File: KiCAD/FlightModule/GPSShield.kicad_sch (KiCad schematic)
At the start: 6 parts

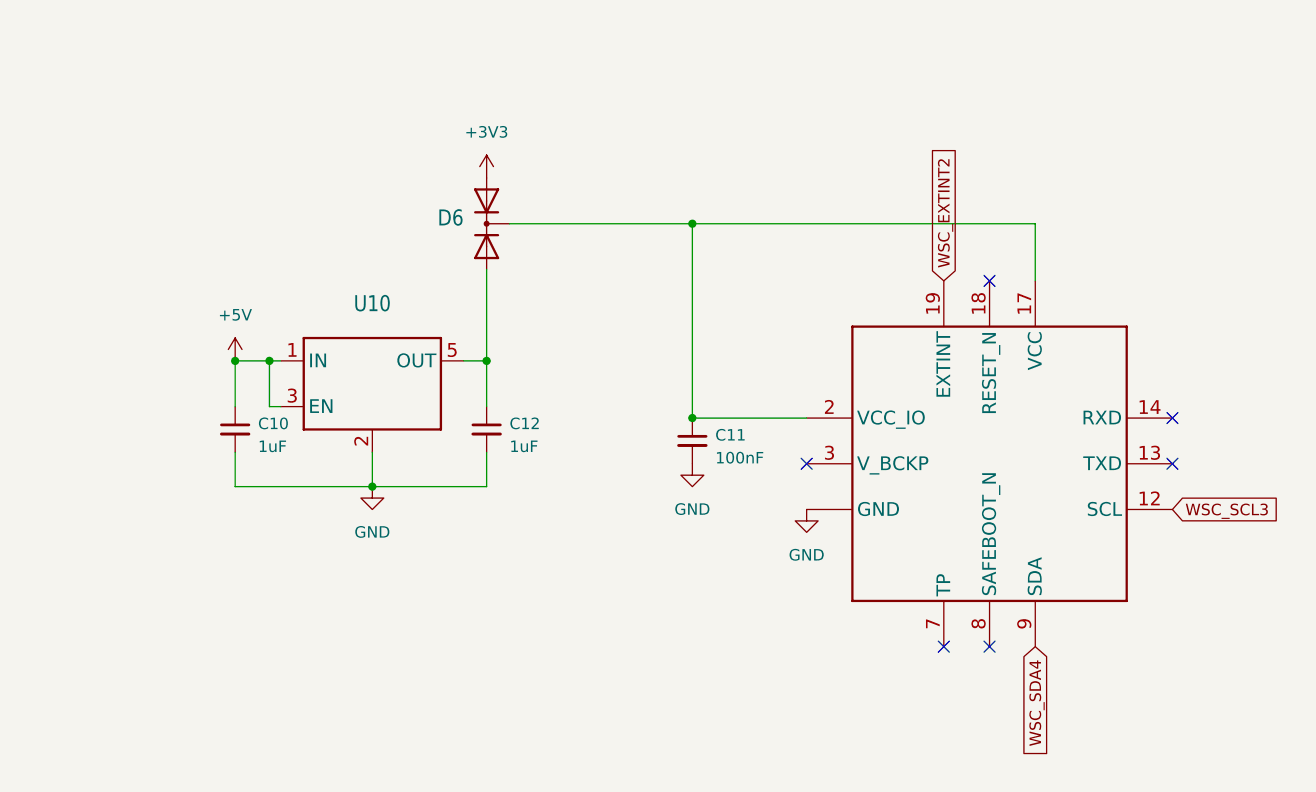
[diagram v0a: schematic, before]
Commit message: GNSSモジュール，SAM-M8Qの回路図完成
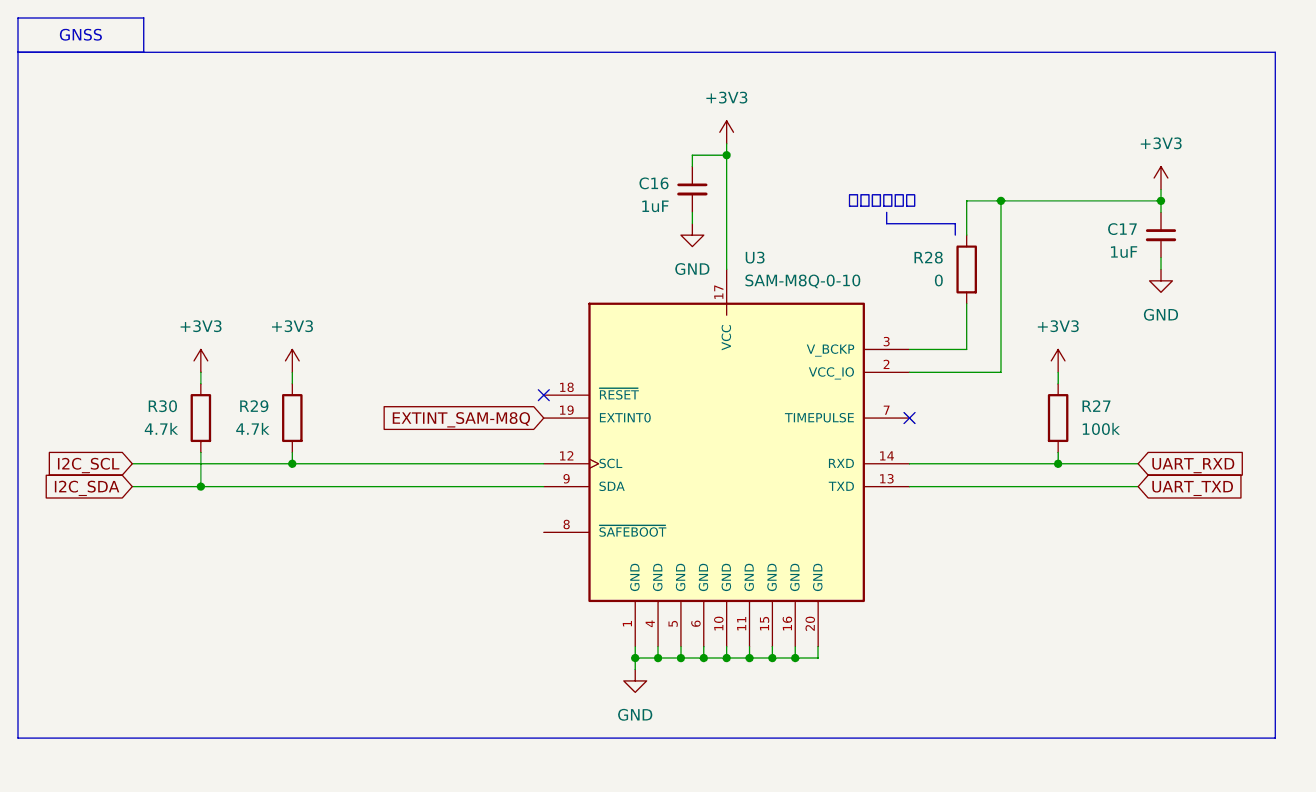
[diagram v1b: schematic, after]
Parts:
- removed C10, C12: 1uF, Capacitor_SMD:C_1206_3216Metric_Pad1.33x1.80mm_HandSolder, symbol Device:C_Small
- removed C11: 100nF, Capacitor_SMD:C_1206_3216Metric_Pad1.33x1.80mm_HandSolder, symbol Device:C_Small
- removed D6: ~, MKRGPSShield_V4.0:SOT65P210X110-3N, symbol MKRGPSShield_V4.0-eagle-import:Arduino-diodes_A2K_SOT-323
- removed IC2: ~, GPSShield:UBLOXLIB_SAM-M8Q, symbol MKRGPSShield_V4.0-eagle-import:SAM-M8Q
- removed U10: ~, MKRGPSShield_V4.0:SOT25, symbol MKRGPSShield_V4.0-eagle-import:AP2112K-3.3
- added C16, C17: 1uF, Capacitor_SMD:C_1206_3216Metric_Pad1.33x1.80mm_HandSolder, symbol Device:C_Small
- added R27: 100k, Resistor_SMD:R_0603_1608Metric_Pad0.98x0.95mm_HandSolder, symbol Device:R
- added R28: 0, Resistor_SMD:R_0603_1608Metric_Pad0.98x0.95mm_HandSolder, symbol Device:R
- added R29, R30: 4.7k, Resistor_SMD:R_0603_1608Metric_Pad0.98x0.95mm_HandSolder, symbol Device:R
- added U3: SAM-M8Q-0-10, TSRP_IC:MODULE_SAM-M8Q-0-10, symbol TSRP_IC:SAM-M8Q-0-10
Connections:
- net +3V3: now also C16.1, C17.1, R27.1, R28.1, R29.1, R30.1, U3.17 (VCC), U3.2 (VCC_IO)
- net GND: now also C16.2, C17.2, U3.1 (GND), U3.10 (GND), U3.11 (GND), U3.15 (GND), U3.16 (GND), U3.20 (GND), U3.4 (GND), U3.5 (GND), U3.6 (GND)
- new net: R28.2, U3.3 (V_BCKP)
- new net EXTINT_SAM-M8Q: U3.19 (EXTINT0)
- new net I2C_SCL: R29.2, U3.12 (SCL)
- new net I2C_SDA: R30.2, U3.9 (SDA)
- new net UART_RXD: R27.2, U3.14 (RXD)
- new net UART_TXD: U3.13 (TXD)
- no-connect marks 6 -> 2
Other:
- note added: "ジャンパ抵抗"

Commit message: 回路図8割完成
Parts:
- U3: footprint TSRP_IC:MODULE_SAM-M8Q-0-10 -> SAM-M8Q-0-10:MODULE_SAM-M8Q-0-10
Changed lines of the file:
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@@
 			)
 		)
-		(property "Footprint" "TSRP_IC:MODULE_SAM-M8Q-0-10"
+		(property "Footprint" "SAM-M8Q-0-10:MODULE_SAM-M8Q-0-10"
 			(at 104.14 68.58 0)
 			(effects
@@
 				(path "/3507137a-fdd7-4bc0-abe8-370b7c3b390e/5f21eb00-60ce-4306-a223-a9b9ec9552df"
 					(reference "#PWR062")
+					(unit 1)
+				)
+			)
+		)
+	)
+	(symbol
+		(lib_name "GND_2")
+		(lib_id "power:GND")
+		(at 93.98 93.98 0)
+		(unit 1)
+		(exclude_from_sim no)
+		(in_bom yes)
+		(on_board yes)
+		(dnp no)
+		(fields_autoplaced yes)
+		(property "Reference" "#PWR014"
+			(at 93.98 100.33 0)
+			(effects
+				(font
+					(size 1.27 1.27)
+				)
+				(hide yes)
+			)
+		)
+		(property "Value" "GND"
+			(at 93.98 99.06 0)
+			(effects
+				(font
+					(size 1.27 1.27)
+				)
+			)
+		)
+		(property "Footprint" ""
+			(at 93.98 93.98 0)
+			(effects
+				(font
+					(size 1.27 1.27)
+				)
+				(hide yes)
+			)
+		)
+		(property "Datasheet" ""
+			(at 93.98 93.98 0)
+			(effects
+				(font
+					(size 1.27 1.27)
+				)
+				(hide yes)
+			)
+		)
+		(property "Description" "Power symbol creates a global label with name \"GND\" , ground"
+			(at 93.98 93.98 0)
+			(effects
+				(font
+					(size 1.27 1.27)
+				)
+				(hide yes)
+			)
+		)
+		(pin "1"
+		)
+		(instances
+			(project "FlightModule"
+				(path "/3507137a-fdd7-4bc0-abe8-370b7c3b390e/5f21eb00-60ce-4306-a223-a9b9ec9552df"
+					(reference "#PWR014")
+					(unit 1)
+				)
+			)
+			(project "GPSShield"
+				(path "/e91f5324-b1bd-4996-81c2-18550b5297b9"
+					(reference "#PWR?")
 					(unit 1)
 				)
@@
 					(unit 1)
 				)
-			)
-		)
-	)
-	(symbol
-		(lib_name "GND_2")
-		(lib_id "power:GND")
-		(at 93.98 93.98 0)
-		(unit 1)
-		(exclude_from_sim no)
-		(in_bom yes)
-		(on_board yes)
-		(dnp no)
-		(fields_autoplaced yes)
-		(property "Reference" "#PWR014"
-			(at 93.98 100.33 0)
-			(effects
-				(font
-					(size 1.27 1.27)
-				)
-				(hide yes)
-			)
-		)
-		(property "Value" "GND"
-			(at 93.98 99.06 0)
-			(effects
-				(font
-					(size 1.27 1.27)
-				)
-			)
-		)
-		(property "Footprint" ""
-			(at 93.98 93.98 0)
-			(effects
-				(font
-					(size 1.27 1.27)
-				)
-				(hide yes)
-			)
-		)
-		(property "Datasheet" ""
-			(at 93.98 93.98 0)
-			(effects
-				(font
-					(size 1.27 1.27)
-				)
-				(hide yes)
-			)
-		)
-		(property "Description" "Power symbol creates a global label with name \"GND\" , ground"
-			(at 93.98 93.98 0)
-			(effects
-				(font
-					(size 1.27 1.27)
-				)
-				(hide yes)
-			)
-		)
-		(pin "1"
-		)
-		(instances
-			(project "FlightModule"
-				(path "/3507137a-fdd7-4bc0-abe8-370b7c3b390e/5f21eb00-60ce-4306-a223-a9b9ec9552df"
-					(reference "#PWR014")
-					(unit 1)
-				)
-			)
-			(project "GPSShield"
-				(path "/e91f5324-b1bd-4996-81c2-18550b5297b9"
-					(reference "#PWR?")
-					(unit 1)
-				)
